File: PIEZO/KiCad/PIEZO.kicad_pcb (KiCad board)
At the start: 2 copper layers, 37 x 32 mm, 8 parts, among them J1 Conn_01x06_Pin

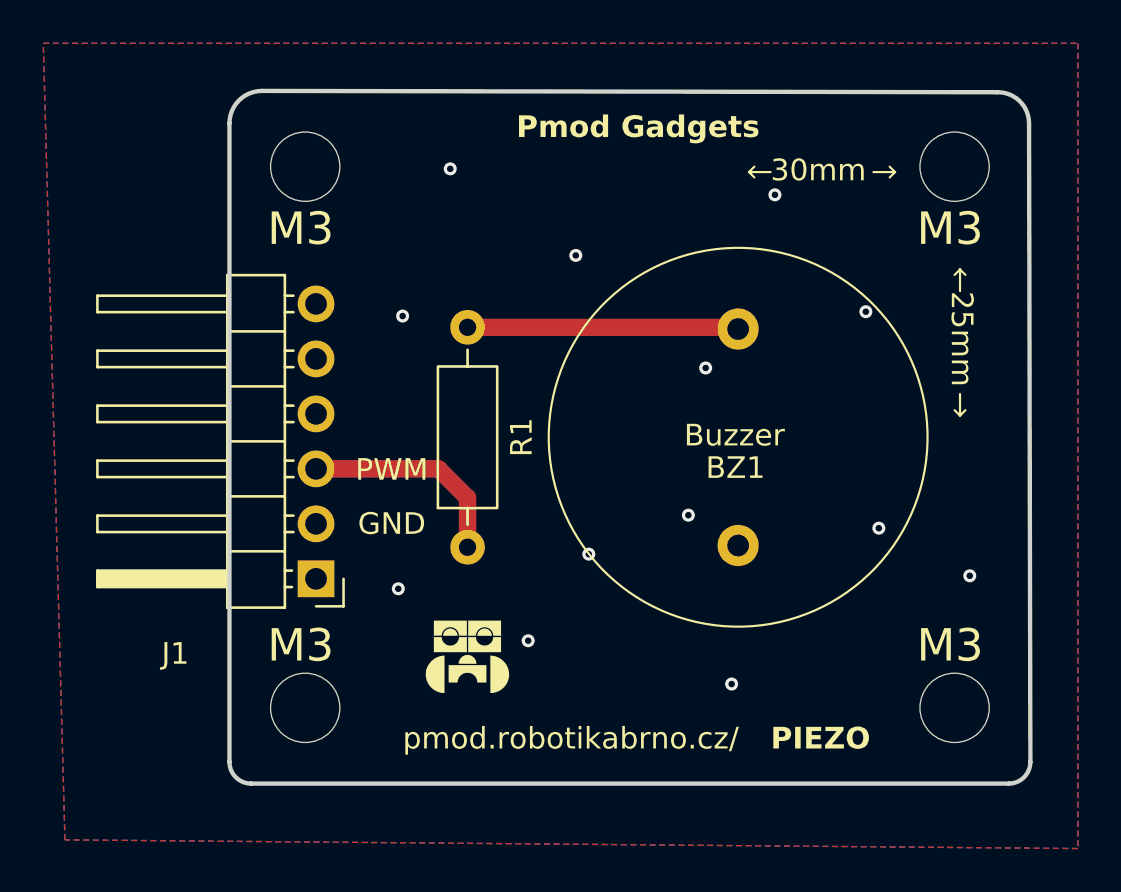
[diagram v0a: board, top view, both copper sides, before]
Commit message: Deployed d972a79 with MkDocs version: 1.6.0
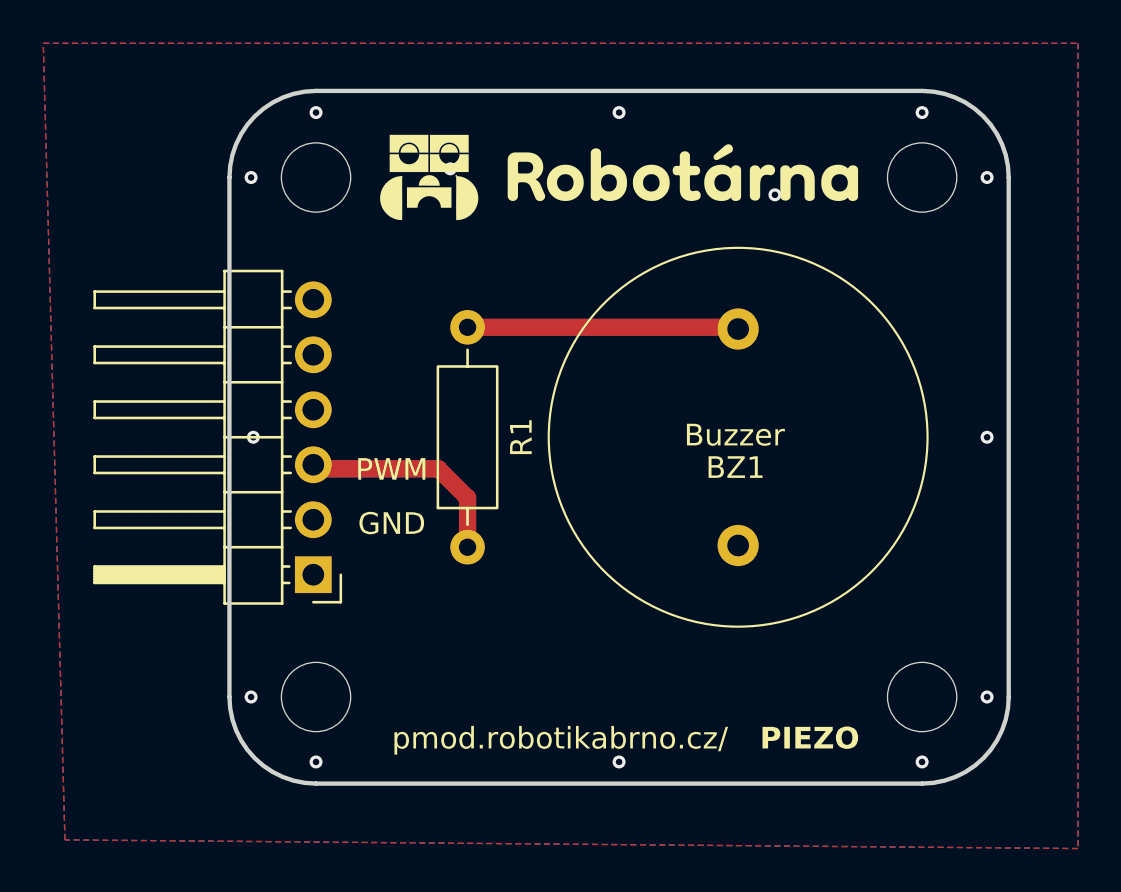
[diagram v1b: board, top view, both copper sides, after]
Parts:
- removed G***: LOGO, LOGO
- moved REF** 1.58 mm to (110.0, 75.0)
- moved REF** 1.58 mm to (110.0, 51.0)
- moved REF** 0.71 mm to (82.0, 75.0)
- moved REF** 0.71 mm to (82.0, 51.0)
- moved J1 0.23 mm to (81.9, 69.3)
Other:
- board size 37 x 32 mm -> 36 x 32 mm
- board text added: "32mm"
- board text added: "36mm"
- board text removed: "25mm"
- board text removed: "30mm"
- board text removed: "M3"
- board text removed: "Pmod Gadgets"
